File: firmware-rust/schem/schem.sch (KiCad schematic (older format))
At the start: 47 parts

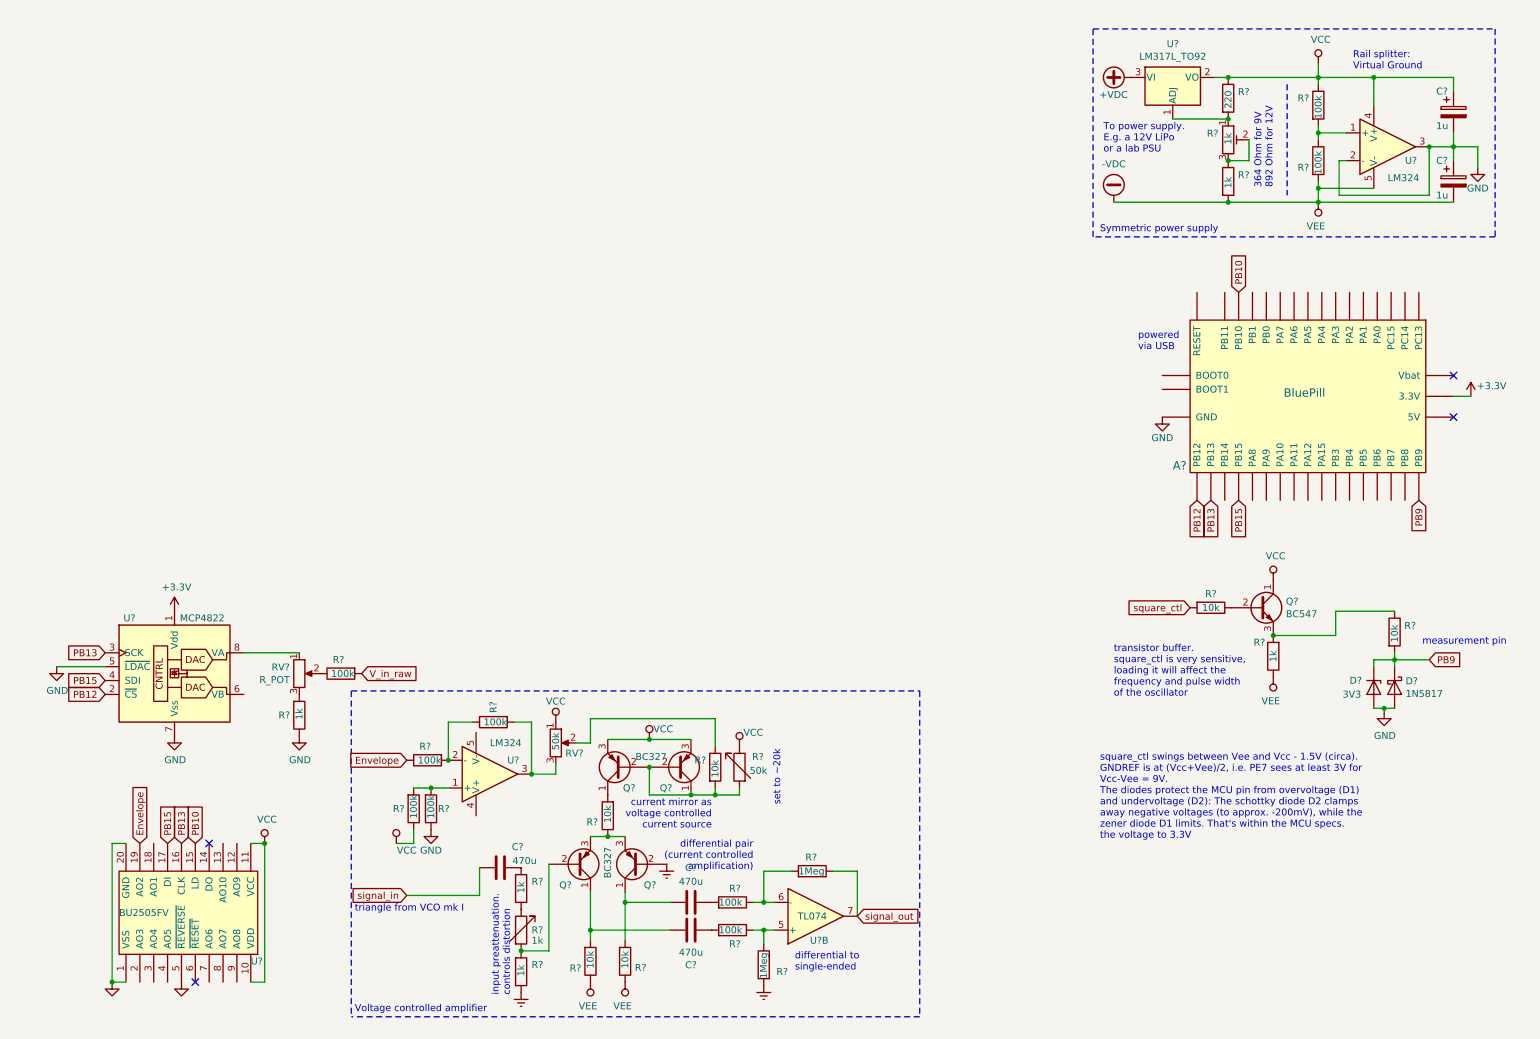
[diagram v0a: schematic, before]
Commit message: working VCF (npn variant)
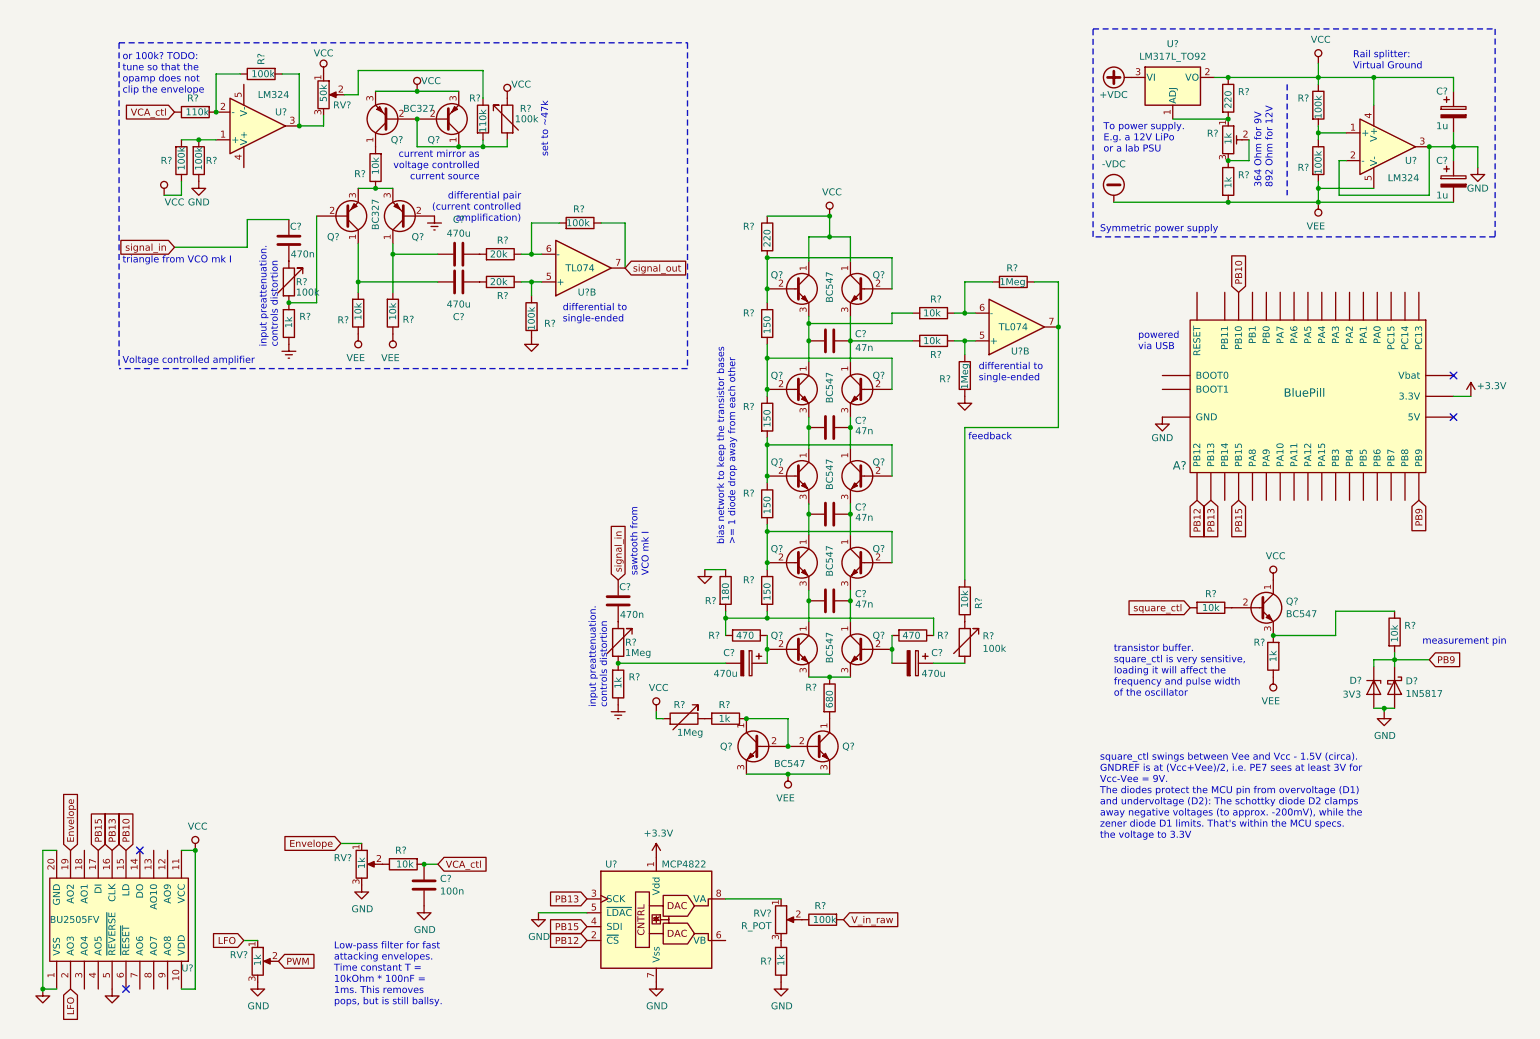
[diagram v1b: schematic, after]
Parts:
- removed R?: 1k, symbol Device:R
- added C?: 100n, symbol Device:C
- added C?: 470n, symbol Device:C
- added C? (x2): 470u, symbol Device:CP
- added C? (x4): 47n, symbol Device:C
- added Q? (x12): BC547, Package_TO_SOT_THT:TO-92_Inline, symbol Transistor_BJT:BC547
- added R? (x4): 10k, symbol Device:R
- added R? (x2): 1k, symbol Device:R
- added R? (x2): 1Meg, symbol Device:R_Variable
- added R? (x4): 150, symbol Device:R
- added R?: 220, symbol Device:R
- added R? (x2): 470, symbol Device:R
- added R?: 180, symbol Device:R
- added R? (x2): 1Meg, symbol Device:R
- added R?: 100k, symbol Device:R_Variable
- added R?: 680, symbol Device:R
- added RV? (x2): 1k, symbol Device:R_POT
- added U?: TL074, symbol Amplifier_Operational:TL074
- C?: value 470u -> 470n
- R?: value 1k -> 100k
- R?: value 10k -> 110k
- R?: value 50k -> 100k
- R?: value 100k -> 110k
- R? (x2): value 100k -> 20k
- R? (x2): value 1Meg -> 100k
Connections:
- net -VDC: now also Q?.3 (E), Q?.3 (E)
- net Envelope: now also RV?.1; no longer R?.1
- net GND: now also R?.2, C?.2, R?.1, R?.2, RV?.3, RV?.3
- net GNDREF: now also R?.1; no longer R?.2
- net VCC: now also Q?.1 (C), Q?.1 (C), R?.1, R?.2
- net signal_in: now also C?.1, C?.1; no longer C?.2
- net at R?.1: now also C?.2
- net LFO: now reaches U?.2 (AO3)
- net LFO: now also RV?.1
- new net: R?.1, RV?.2
- new net: C?.2, R?.1
- new net: C?.2, R?.2, R?.2
- new net: C?.1, Q?.2 (B), R?.1
- new net: C?.1, Q?.1 (C), Q?.3 (E) (x3)
- new net: C?.2, Q?.1 (C), Q?.3 (E) (x3)
- new net: Q?.2 (B), Q?.2 (B), R?.1, R?.2 (x4)
- new net: C?.2, Q?.1 (C), Q?.3 (E), R?.2
- new net: C?.1, Q?.1 (C), Q?.3 (E), R?.2
- new net: C?.2, Q?.2 (B), R?.2
- new net: Q?.3 (E), Q?.3 (E), R?.1
- new net: R?.1, R?.2, R?.2, R?.2
- new net: R?.1, R?.1, U?.5 (+)
- new net: R?.1, R?.2, U?.6 (-)
- new net: R?.1, R?.2, U?.7
- new net: R?.1, R?.1
- new net: C?.1, R?.2
- new net: Q?.1 (C), R?.2
- new net: Q?.1 (C), Q?.2 (B), Q?.2 (B), R?.1
- new net: R?.1, R?.2
- new net PWM: RV?.2
- new net VCA_ctl: C?.1, R?.1, R?.2
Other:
- note added: "Low-pass filter for fast\nattacking envelopes.\nTime constant T =\n10kOhm * 100nF = \n1ms. This removes\npops, but is still ballsy."
- note added: "bias network to keep the transistor bases\n>= 1 diode drop away from each other"
- note added: "feedback"
- note added: "or 100k? TODO:\ntune so that the\nopamp does not\nclip the envelope"
- note added: "sawtooth from\nVCO mk I"
- note added: "set to ~~47k"
- note removed: "set to ~~20k"
- moved on the sheet: C?, Q?, R?, RV?, U?, U?B

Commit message: VCF with pnp
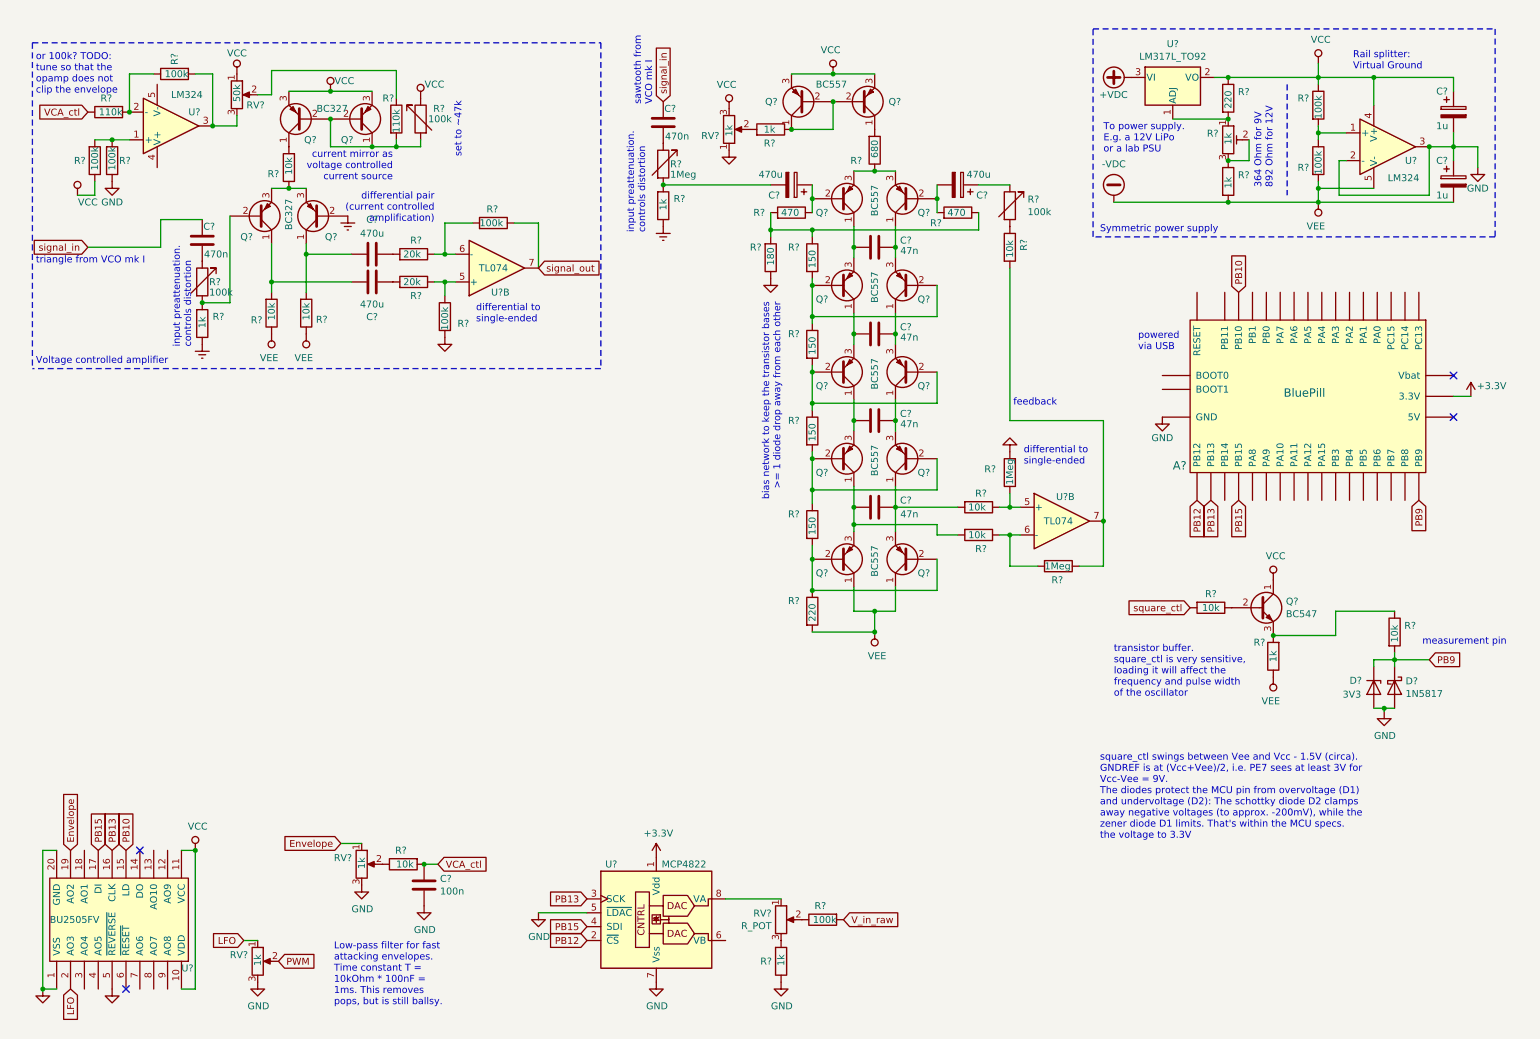
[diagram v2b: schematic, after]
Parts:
- removed Q? (x12): BC547, Package_TO_SOT_THT:TO-92_Inline, symbol Transistor_BJT:BC547
- removed R?: 1Meg, symbol Device:R_Variable
- added Q? (x12): BC557, Package_TO_SOT_THT:TO-92_Inline, symbol Transistor_BJT:BC557
- added RV?: 1k, symbol Device:R_POT
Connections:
- net -VDC: now also R?.2, Q?.1 (C), Q?.1 (C)
- net GND: now also RV?.1
- net VCC: now also Q?.3 (E), Q?.3 (E), RV?.3; no longer R?.1
- net at C?.1, R?.1: now also Q?.2 (B)
- net at C?.1: now also Q?.1 (C), Q?.3 (E) (x3)
- net at C?.2: now also Q?.1 (C), Q?.3 (E) (x3)
- net at R?.2: now also R?.1, Q?.2 (B), Q?.2 (B); no longer R?.1 (x3)
- net at C?.2, R?.2: now also Q?.1 (C), Q?.3 (E)
- net at C?.1, R?.2: now also Q?.1 (C), Q?.3 (E)
- net at C?.2, R?.2: now also Q?.2 (B)
- net at R?.1: now also Q?.3 (E), Q?.3 (E)
- net at R?.1, R?.2, R?.2: now also R?.1; no longer R?.2
- net at R?.1: now also R?.2; no longer R?.1
- net at C?.1: now also R?.1; no longer R?.2
- net at R?.2: now also Q?.1 (C)
- net at R?.1: now also Q?.1 (C), Q?.2 (B), Q?.2 (B)
- net at R?.2: now also RV?.2
- new net: Q?.2 (B), Q?.2 (B), R?.1, R?.2
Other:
- moved on the sheet: C?, Q?, R?, RV?, U?, U?B
